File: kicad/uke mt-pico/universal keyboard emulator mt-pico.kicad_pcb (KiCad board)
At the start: 2 copper layers, 42 parts, among them J1 Mode Select, J2 OLED Adapter, J3 Serial, J4 Conn_02x20_Odd_Even, J5 SWD, J6 Pico VBUS, SW1 Reset Pico, U1 MT8816, U2 74HCT245, U3 74HCT245, U4 Pico, U5 74HCT595-VERIFY-FOOTPRINT

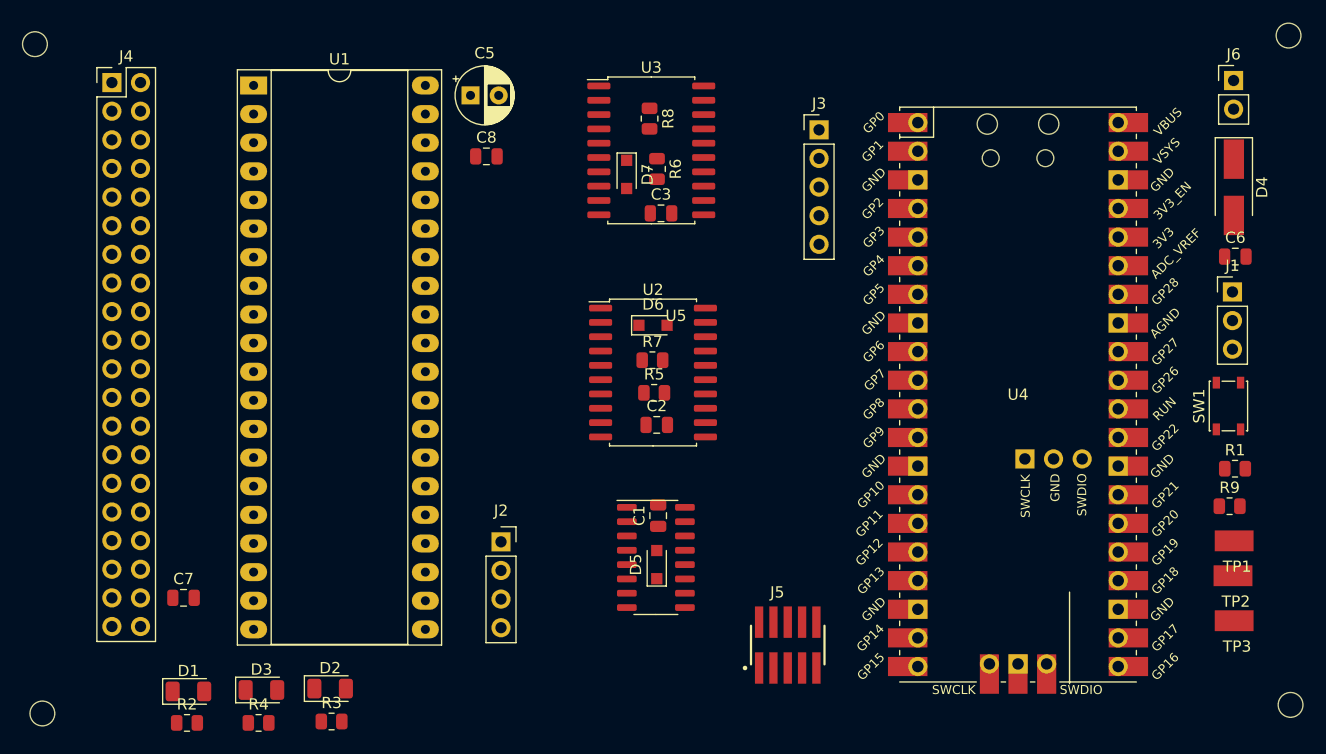
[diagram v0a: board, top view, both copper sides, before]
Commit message: minor pixel pushing
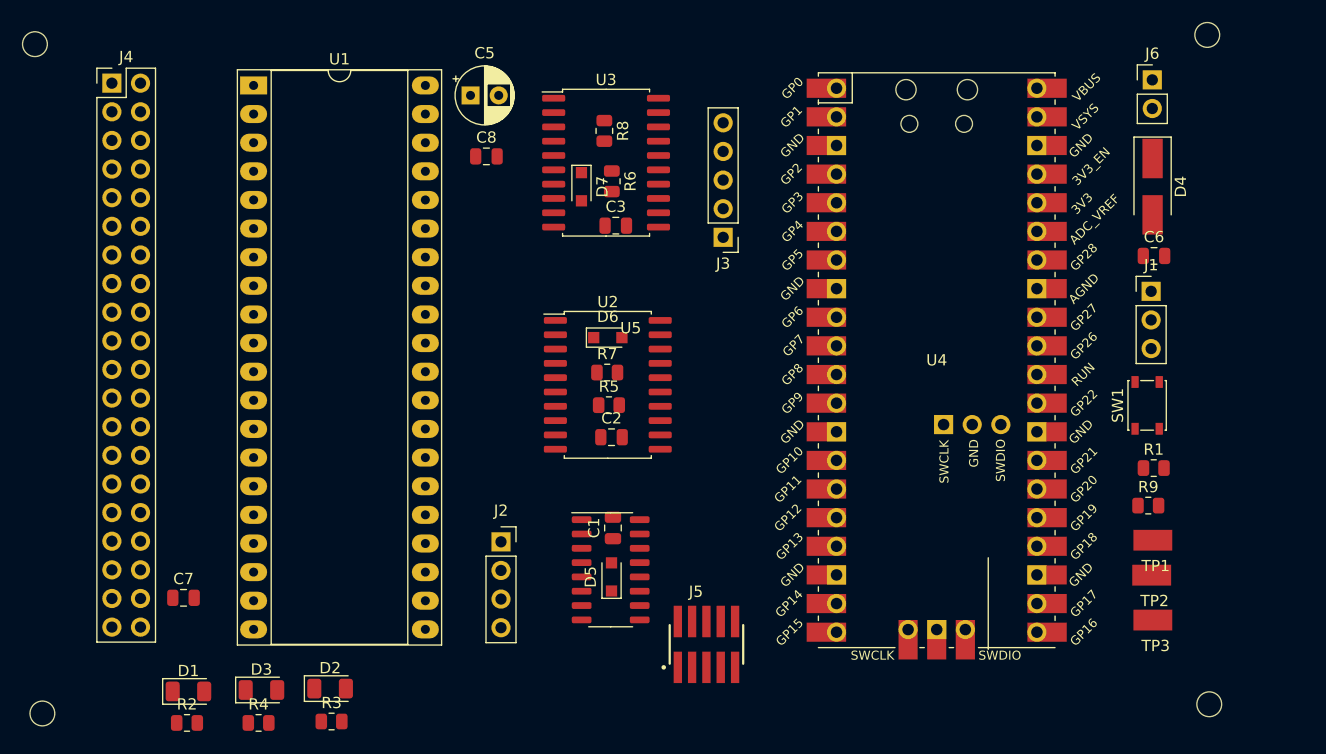
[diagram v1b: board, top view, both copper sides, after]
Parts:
- moved J3 12.8 mm to (166.9, 74.1), turned to 180 degrees
- moved U4 7.83 mm to (185.8, 85.0)
- moved C6 7.21 mm to (205.1, 75.7)
- moved H2 7.21 mm to (209.8, 56.1)
- moved J1 7.21 mm to (204.9, 78.9)
- moved J5 7.21 mm to (165.4, 110.2)
- moved J6 7.21 mm to (205.0, 60.1)
- moved R1 7.21 mm to (205.1, 94.5)
- moved SW1 7.21 mm to (204.5, 89.0)
- moved TP1 7.21 mm to (205.0, 100.9)
- moved TP3 7.21 mm to (205.0, 108.0)
- moved D4 7.21 mm to (205.0, 69.6)
- moved H4 7.21 mm to (210.0, 115.5)
- moved R9 7.21 mm to (204.6, 97.9)
- moved TP2 7.21 mm to (204.9, 104.0)
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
